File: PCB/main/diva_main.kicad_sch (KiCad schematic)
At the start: 66 parts, among them J1 Conn_01x04, K1 Conn_01x01_Female, K10 Conn_01x01_Female, K11 Conn_01x01_Female, K12 Conn_01x01_Female, K13 Conn_01x01_Female, K14 Conn_01x01_Female, K15 Conn_01x01_Female, K16 Conn_01x01_Female, K2 Conn_01x01_Female, K3 Conn_01x01_Female, K4 Conn_01x01_Female, K5 Conn_01x01_Female, K6 Conn_01x01_Female, K7 Conn_01x01_Female, K8 Conn_01x01_Female, K9 Conn_01x01_Female, SW1 SWITCH_SPST, SW2 SWITCH_SPST, SW3 SWITCH_SPST, SW4 SWITCH_SPST, SW5 SWITCH_SPST, SW6 SWITCH_SPST, SW7 SWITCH_SPST, U1 Pico_Trim, U2 MPR121QR2_BOARD, U3 MPR121QR2_BOARD, U8 SN74LV1T34DBV

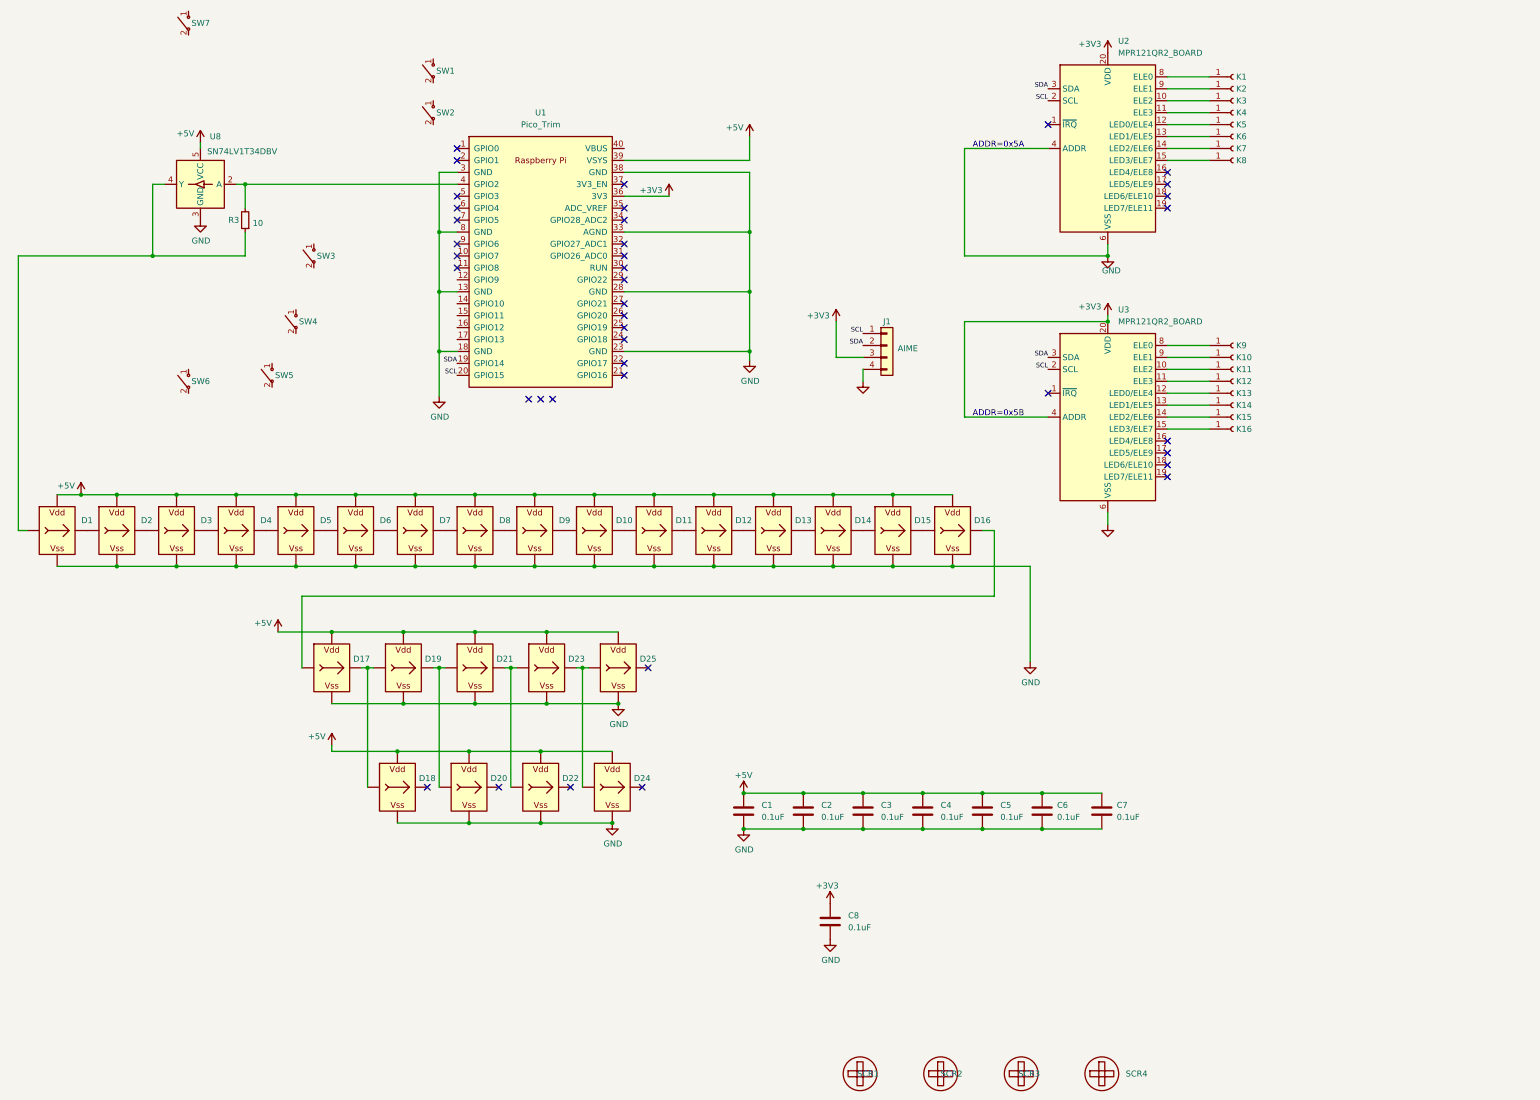
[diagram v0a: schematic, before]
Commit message: PCB v1.0 ready
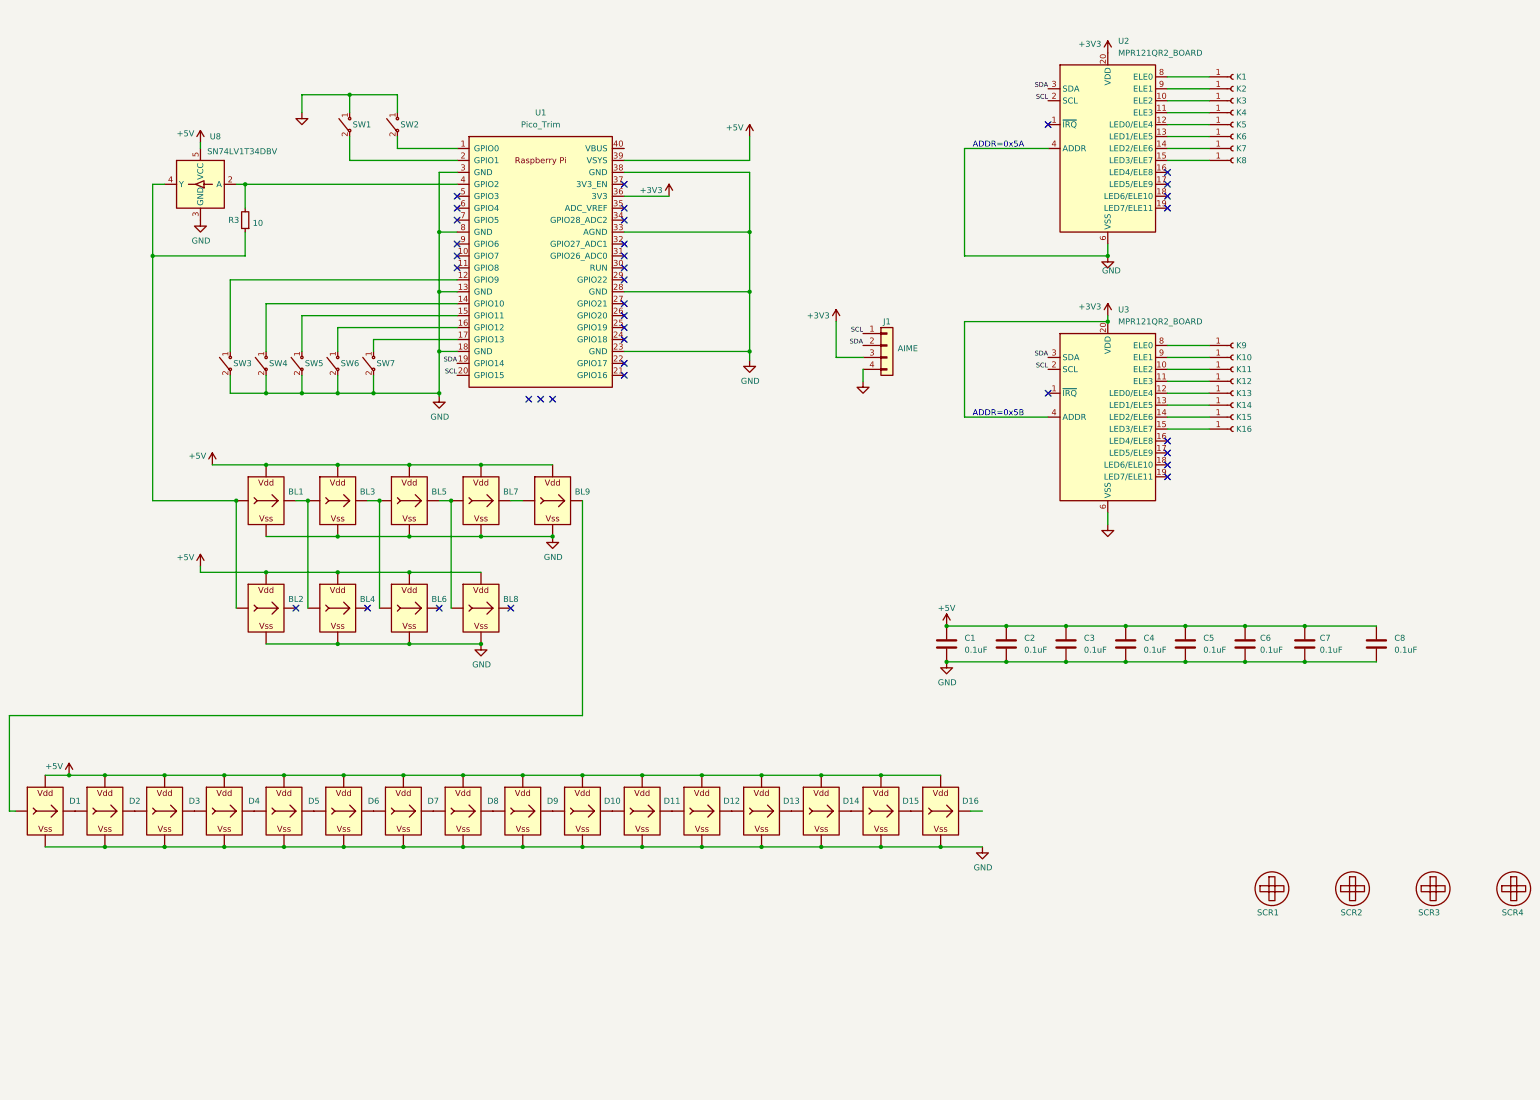
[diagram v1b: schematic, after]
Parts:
- renumbered D17 to BL1, D18 to BL2, D19 to BL3, D20 to BL4, D21 to BL5, D22 to BL6, D23 to BL7, D24 to BL8, D25 to BL9
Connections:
- net +3V3: no longer C8.1
- net +5V: now also C8.1
- net GND: now also SW1.1 ("~{"}), SW2.1 ("~{"}), SW3.2 ("~{"}), SW4.2 ("~{"}), SW5.2 ("~{"}), SW6.2 ("~{"}), SW7.2 ("~{"})
- net at SW4.1 ("~{"}): now also U1.14 (GPIO10)
- net at BL7.O (Out), BL9.I (In): no longer BL8.I (In)
- net at BL3.O (Out), BL5.I (In): now also BL6.I (In); no longer BL4.I (In)
- net at BL5.O (Out), BL7.I (In): now also BL8.I (In); no longer BL6.I (In)
- net at R3.1, U8.4 (Y): now also BL1.I (In), BL2.I (In); no longer D1.I (In)
- net at U1.1 (GPIO0): now also SW2.2 ("~{"})
- net at U1.12 (GPIO9): now also SW3.1 ("~{"})
- net at U1.15 (GPIO11): now also SW5.1 ("~{"})
- net at U1.16 (GPIO12): now also SW6.1 ("~{"})
- net at U1.17 (GPIO13): now also SW7.1 ("~{"})
- net at U1.2 (GPIO1): now also SW1.2 ("~{"})
- net at BL9.O (Out): now also D1.I (In)
- net at BL1.O (Out), BL3.I (In): now also BL4.I (In); no longer BL2.I (In)
- net at D16.O (Out): no longer BL1.I (In)
- no-connect marks 39 -> 36
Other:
- moved on the sheet: BL1, BL2, BL3, BL4, BL5, BL6, BL7, BL8, BL9, C1, C2, C3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
